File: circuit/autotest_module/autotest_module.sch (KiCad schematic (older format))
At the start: 9 parts, among them K1 ACC_Relay_Module, K2 Rev_Relay_Module, U1 ESP32-WROOM-32, U1 PS2561A, U2 INA219-ina219, U2 PS2561A, U3 SSD1306_OLED_0.96

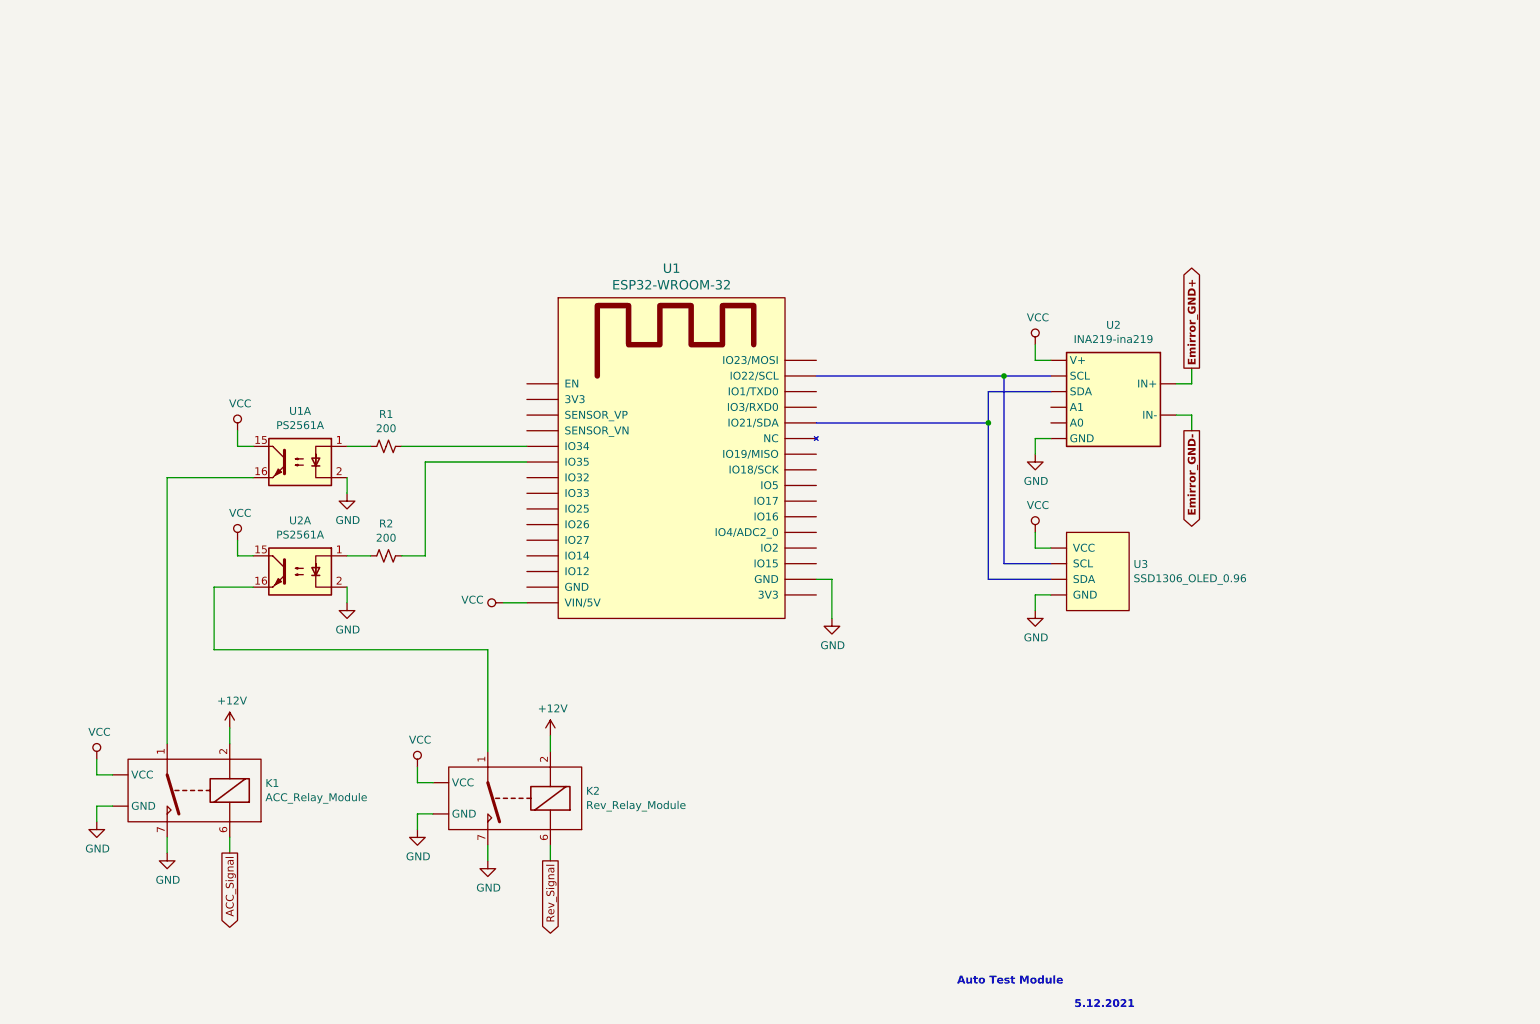
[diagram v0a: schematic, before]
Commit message: update layout
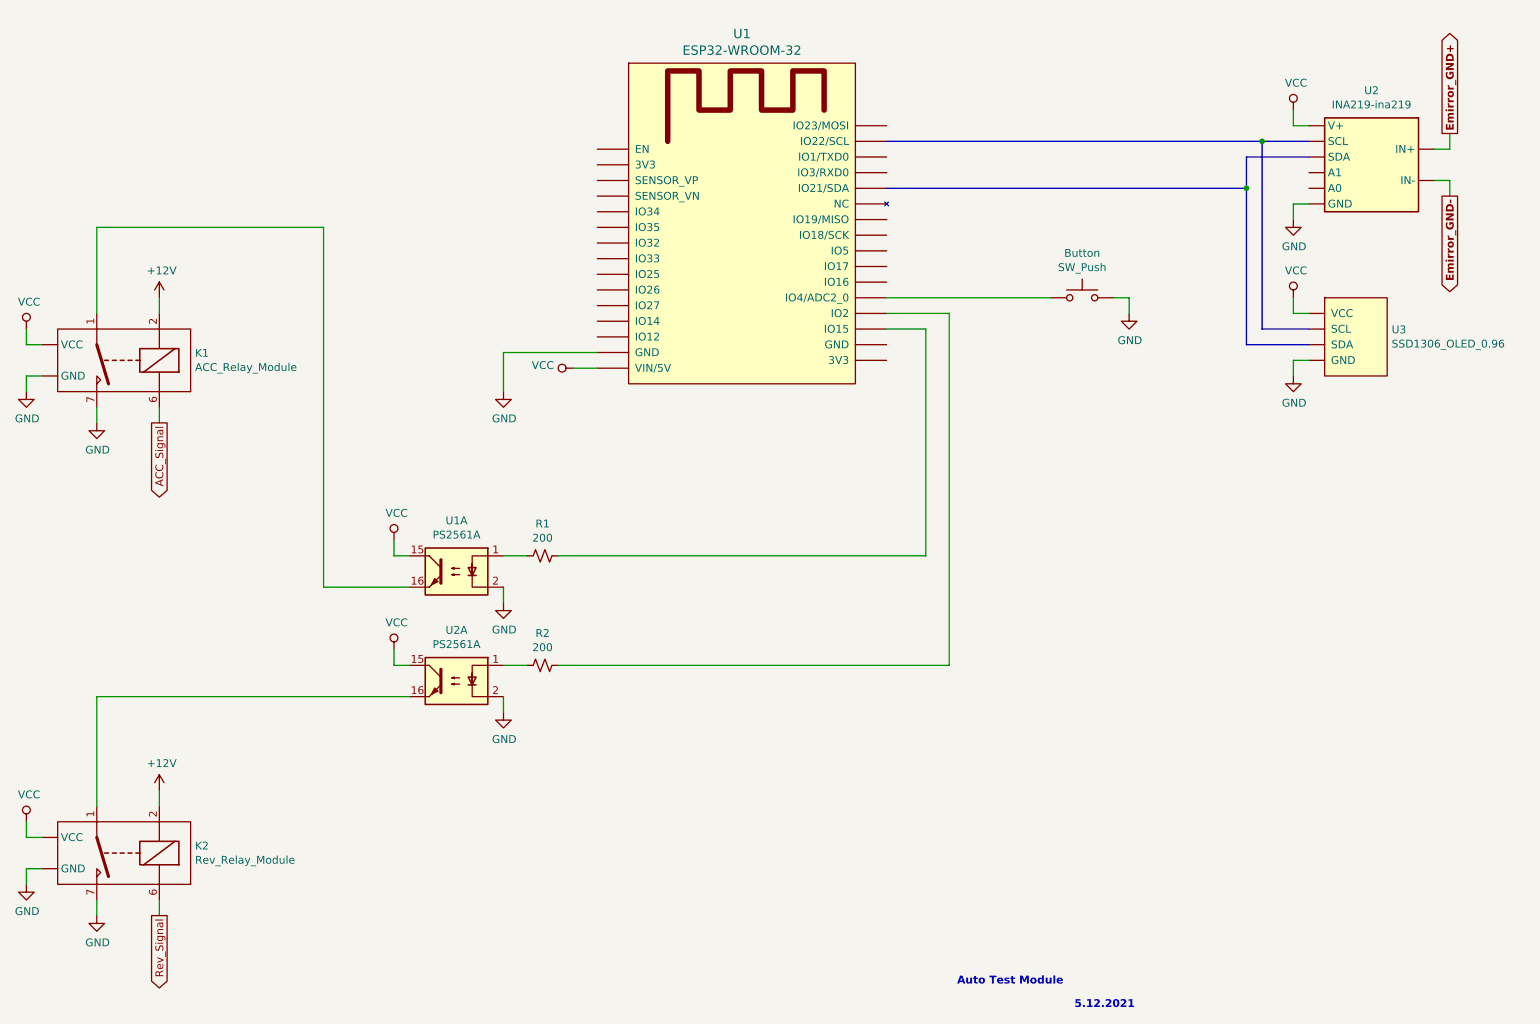
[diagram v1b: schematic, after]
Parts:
- added Button: SW_Push, symbol Switch:SW_Push
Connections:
- net GND: now also U1.1 (GND), Button.2; no longer U1.~ (VIN/5V)
- net at U1.24 (IO2): now also R2.2
- net at U1.26 (IO4/ADC2_0): now also Button.1
- net at U1.6 (IO34): no longer R1.2
- net at U1.7 (IO35): no longer R2.2
- new net: R1.2, U1.~ (VIN/5V)
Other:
- moved on the sheet: K1, K2, R1, R2, U1, U1A, U2, U2A, U3
